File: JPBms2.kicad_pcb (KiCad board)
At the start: 4 copper layers, 69 x 39 mm, 88 parts, among them J1 Conn_ARM_SWD_TagConnect_TC2030, J2 Barrel_Jack_MountingPin, Q1 AO3401A, Q10 AO3401A, Q11 2N7002, Q2 AO3401A, Q3 AO3400A, Q4 AO3400A, Q5 AO3401A, Q6 2N7002, Q7 2N7002, Q8 AO3401A, U1 ST715M25R, U2 STM32L053R8Tx, U3 ZXCT1107, U4 IRS2003, U5 IRS2003

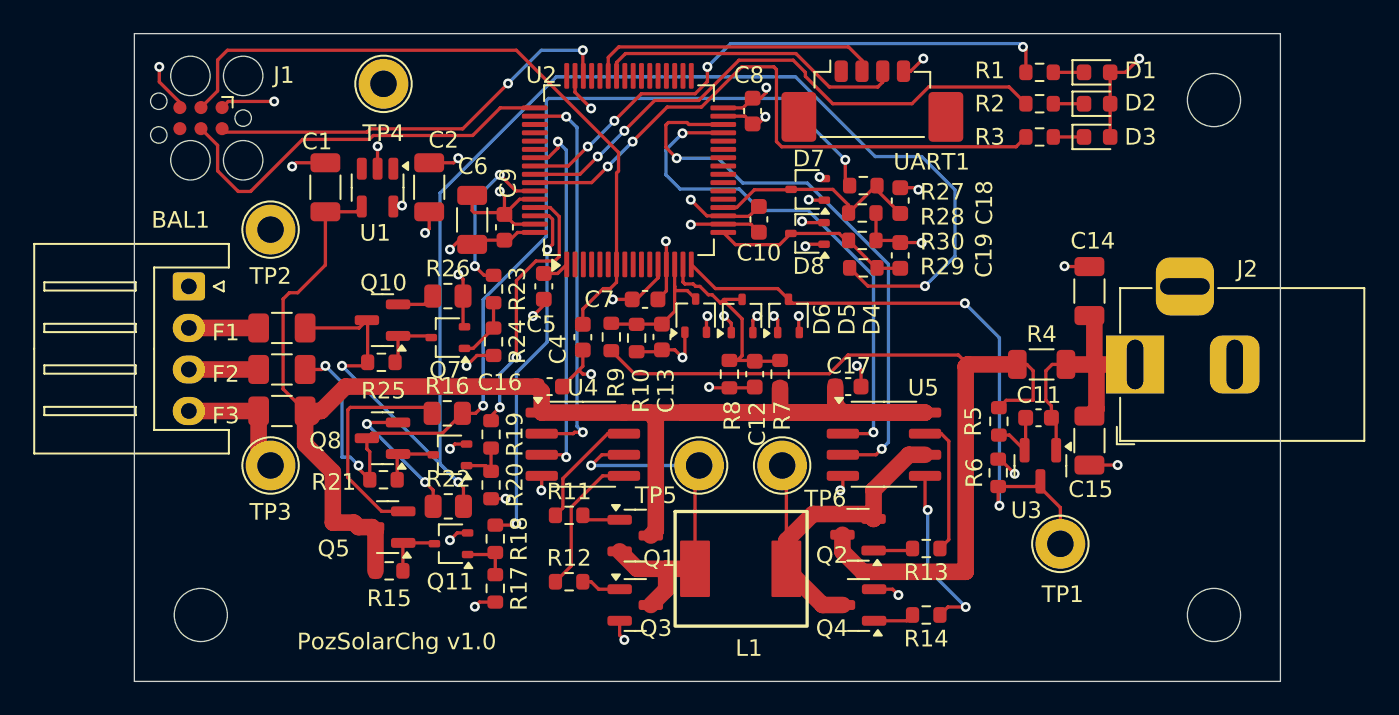
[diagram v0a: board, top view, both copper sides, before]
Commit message: New design and layout
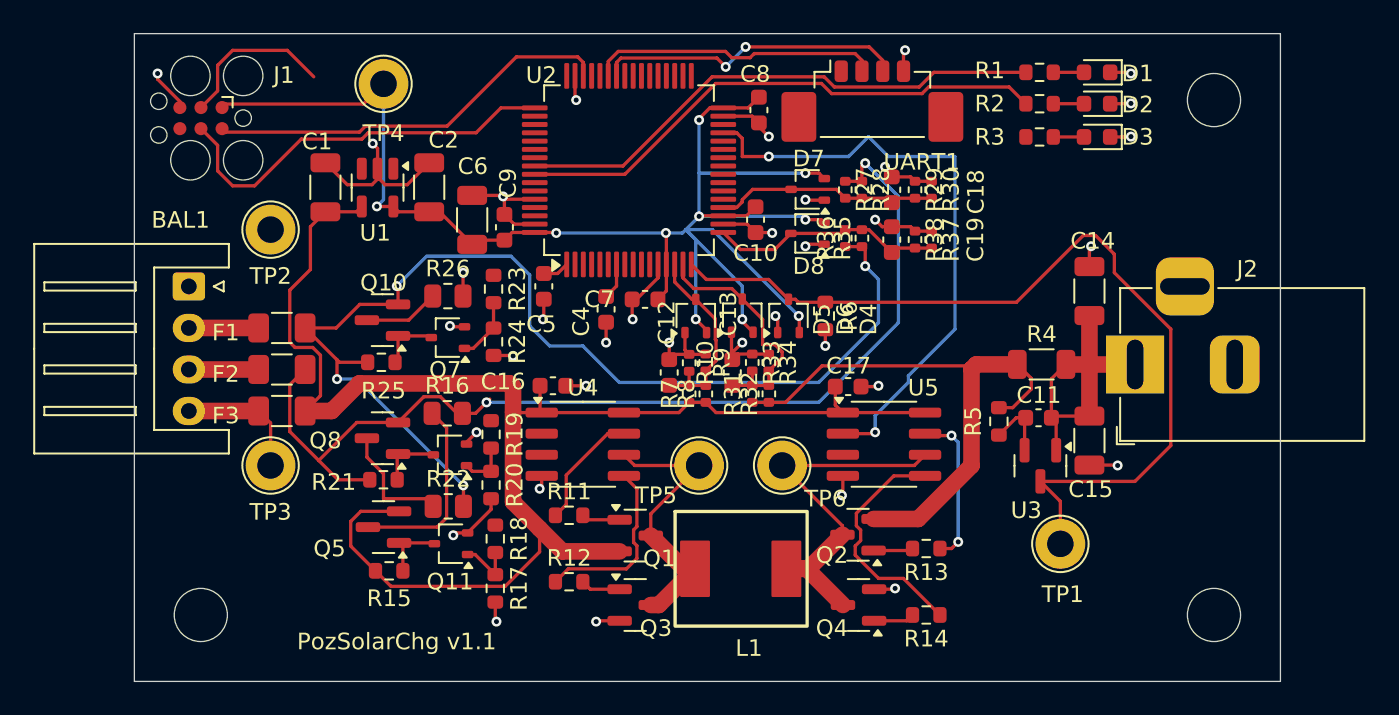
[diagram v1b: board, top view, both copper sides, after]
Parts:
- added R31: 220k, Resistor_SMD:R_0402_1005Metric, F.Cu at (133.2, 83.7)
- added R32: 220k, Resistor_SMD:R_0402_1005Metric, F.Cu at (134.2, 83.7)
- added R33: 47.5k, Resistor_SMD:R_0402_1005Metric, F.Cu at (133.2, 81.8)
- added R34: 47.5k, Resistor_SMD:R_0402_1005Metric, F.Cu at (134.2, 81.8)
- added R35: 220k, Resistor_SMD:R_0402_1005Metric, F.Cu at (139.8, 74.3)
- added R36: 220k, Resistor_SMD:R_0402_1005Metric, F.Cu at (138.8, 74.3)
- added R37: 47.5k, Resistor_SMD:R_0402_1005Metric, F.Cu at (144.0, 74.4)
- added R38: 47.5k, Resistor_SMD:R_0402_1005Metric, F.Cu at (143.0, 74.4)
- BAL1: value Conn_01x04 -> Conn_01x04 JST-XH
- C12, C13, C18, C19: value 1n -> .1u
- D1: value LED -> LED_G
- D2: value LED -> LED_Y
- D3: value LED -> LED_R
- R10: value 39k -> 47.5k; footprint Resistor_SMD:R_0603_1608Metric -> Resistor_SMD:R_0402_1005Metric
- R27: value 390k -> 220k; footprint Resistor_SMD:R_0603_1608Metric -> Resistor_SMD:R_0402_1005Metric
- R28: value 150k -> 220k; footprint Resistor_SMD:R_0603_1608Metric -> Resistor_SMD:R_0402_1005Metric
- R29: value 150k -> 47.5k; footprint Resistor_SMD:R_0603_1608Metric -> Resistor_SMD:R_0402_1005Metric
- R30, R9: value 200k -> 47.5k; footprint Resistor_SMD:R_0603_1608Metric -> Resistor_SMD:R_0402_1005Metric
- R4: value 0.25 -> 0.1
- R6: value 1.2k -> 3k
- R7: value 200k -> 220k; footprint Resistor_SMD:R_0603_1608Metric -> Resistor_SMD:R_0402_1005Metric
- R8: value 39k -> 220k; footprint Resistor_SMD:R_0603_1608Metric -> Resistor_SMD:R_0402_1005Metric
- UART1: value Conn_01x04 -> Conn_01x04 Picoblade
- moved R6 14.1 mm to (137.6, 79.0), turned to -90 degrees
- moved R9 5.89 mm to (130.4, 81.8), turned to -90 degrees
- moved R29 5.64 mm to (143.0, 71.4), turned to -90 degrees
- moved R7 5.60 mm to (129.4, 83.7)
- moved R30 5.17 mm to (144.0, 71.4), turned to -90 degrees
- moved C12 5.15 mm to (128.2, 82.4), turned to 90 degrees
- moved C13 4.75 mm to (132.0, 82.4), turned to 90 degrees
- moved R10 3.50 mm to (129.4, 81.8), turned to -90 degrees
- moved D6 2.81 mm to (132.6, 79.0)
- moved D5 2.79 mm to (129.8, 79.0)
- moved C4 2.18 mm to (124.4, 78.6)
- moved R8 1.85 mm to (130.4, 83.7)
- moved R28 1.40 mm to (139.8, 71.4), turned to -90 degrees
- moved R27 1.12 mm to (138.8, 71.4), turned to -90 degrees
- moved C19 1.08 mm to (141.6, 74.4)
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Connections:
- D1 pad 1: Net-(D1-K) -> GND
- D1 pad 2: VDD -> Net-(D1-A)
- D2 pad 1: Net-(D2-K) -> GND
- D2 pad 2: VDD -> Net-(D2-A)
- D3 pad 1: Net-(D3-K) -> GND
- D3 pad 2: VDD -> Net-(D3-A)
- Q1 pad 2: /BuckBoost/VS_A -> +BATT
- Q1 pad 3: +BATT -> /BuckBoost/VS_A
- Q10 pad 2: Net-(Q10-S) -> CELL_4V
- Q10 pad 3: CELL_4V -> Net-(Q10-D)
- Q2 pad 2: /BuckBoost/VS_B -> VSOLAR
- Q2 pad 3: VSOLAR -> /BuckBoost/VS_B
- Q5 pad 2: Net-(Q5-S) -> +BATT
- Q5 pad 3: +BATT -> Net-(Q5-D)
- Q8 pad 2: Net-(Q8-S) -> CELL_8V
- Q8 pad 3: CELL_8V -> Net-(Q8-D)
- R1 pad 2: Net-(D1-K) -> Net-(D1-A)
- R10 pad 2: VSOLAR_ADC -> VBATT_ADC
- R16 pad 1: Net-(Q5-S) -> Net-(Q5-D)
- R2 pad 2: Net-(D2-K) -> Net-(D2-A)
- R22 pad 1: Net-(Q8-S) -> Net-(Q8-D)
- R26 pad 1: Net-(Q10-S) -> Net-(Q10-D)
- R28 pad 1: GND -> CELL_8V
- R29 pad 1: CELL_4V -> GND
- R29 pad 2: CELL_4V_ADC -> CELL_8V_ADC
- R3 pad 2: Net-(D3-K) -> Net-(D3-A)
- R30 pad 2: CELL_4V_ADC -> CELL_8V_ADC
- R8 pad 1: GND -> +BATT
- R9 pad 1: VSOLAR -> GND
- R9 pad 2: VSOLAR_ADC -> VBATT_ADC
- U2 pad 14: VSOLAR_ADC -> VBATT_ADC
- U2 pad 15: VBATT_ADC -> VSOLAR_ADC
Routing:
- net VDD: track 34.3 -> 96.7 mm, vias 13 -> 10
- net /MCU/LED_ERROR: track 37.2 -> 0.00 mm, vias 2 -> 0
- net DD_BOT_B: track 35.0 -> 0.00 mm, vias 2 -> 0
- net /MCU/NRST: track 41.7 -> 12.0 mm
- net DD_TOP_A: track 23.8 -> 0.00 mm, vias 2 -> 0
- net DD_BOT_A: track 22.8 -> 0.00 mm, vias 2 -> 0
- net NBAL_3: track 21.7 -> 0.00 mm, vias 2 -> 0
- net CELL_4V: track 85.7 -> 66.8 mm, vias 3 -> 4
- net VSOLAR: track 52.3 -> 34.6 mm
- net NBAL_2: track 16.4 -> 0.00 mm, vias 2 -> 0
- net SOLAR_CURRENT_ADC: track 38.6 -> 54.5 mm, vias 2 -> 0
- net Net-(Q5-S): track 13.5 -> 0.00 mm
- net Net-(Q5-D): track 0.00 -> 11.6 mm
- net NBAL_1: track 9.98 -> 0.00 mm, vias 2 -> 0
- net Net-(Q8-S): track 8.52 -> 0.00 mm, vias 2 -> 0
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- added copper zone on In2.Cu, net GND
- removed copper zone on In2.Cu, net VDD
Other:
- board text added: "PozSolarChg v1.1"
- board text removed: "PozSolarChg v1.0"
